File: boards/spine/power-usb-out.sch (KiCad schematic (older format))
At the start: 9 parts

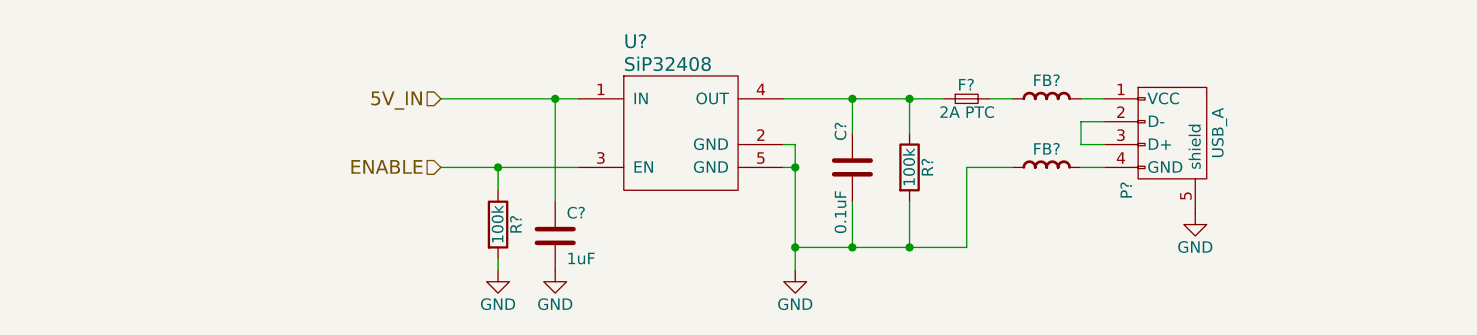
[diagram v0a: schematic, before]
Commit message: Power management and such
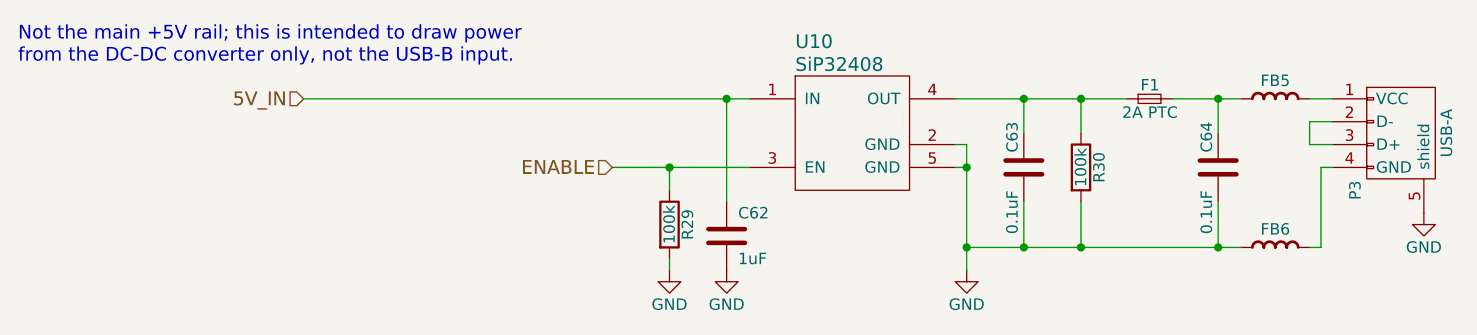
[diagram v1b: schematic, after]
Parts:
- added C64: 0.1uF, 0805, symbol C
- P3: renamed from P?; value USB_A -> USB-A; MfgId (none) -> USB-A1SSW6; MfrId (none) -> On-Shore Tech; RefPrice1k (none) -> 0.35310; Vend1 (none) -> Digikey; Vend1Id (none) -> ED2991-ND
- U10: renamed from U?; MfgId (none) -> Vishay; MfrId (none) -> SIP32408DNP-T1-GE4; RefPrice1k (none) -> 0.175; Vend1 (none) -> Digikey; Vend1Id (none) -> SIP32408DNP-T1-GE4CT-ND
- gave numbers to parts that had none: 7
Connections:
- net GND: now also C64.1
- net at F1.2, FB5.1: now also C64.2
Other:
- note added: "Not the main +5V rail; this is intended to draw power\nfrom the DC-DC converter only, not the USB-B input."
- moved on the sheet: C62, C63, F1, FB5, FB6, P3, R29, R30, U10
